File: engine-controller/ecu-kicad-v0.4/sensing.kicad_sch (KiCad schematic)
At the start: 0 parts

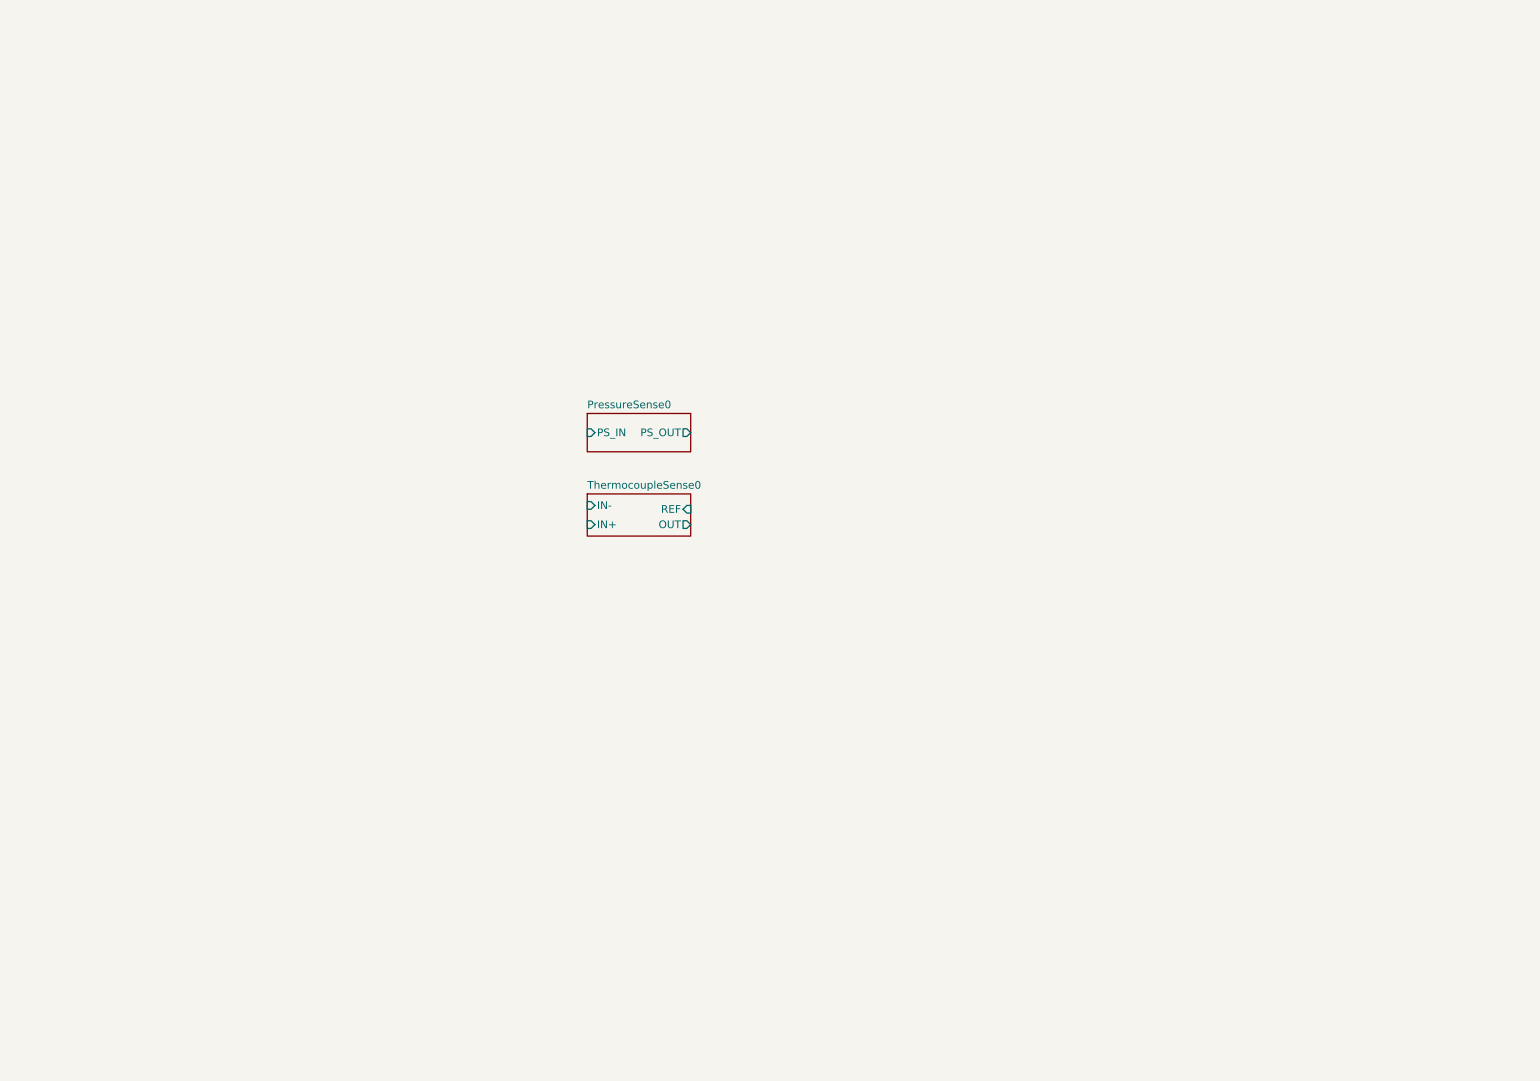
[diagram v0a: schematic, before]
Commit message: Progress on ECU v0.4
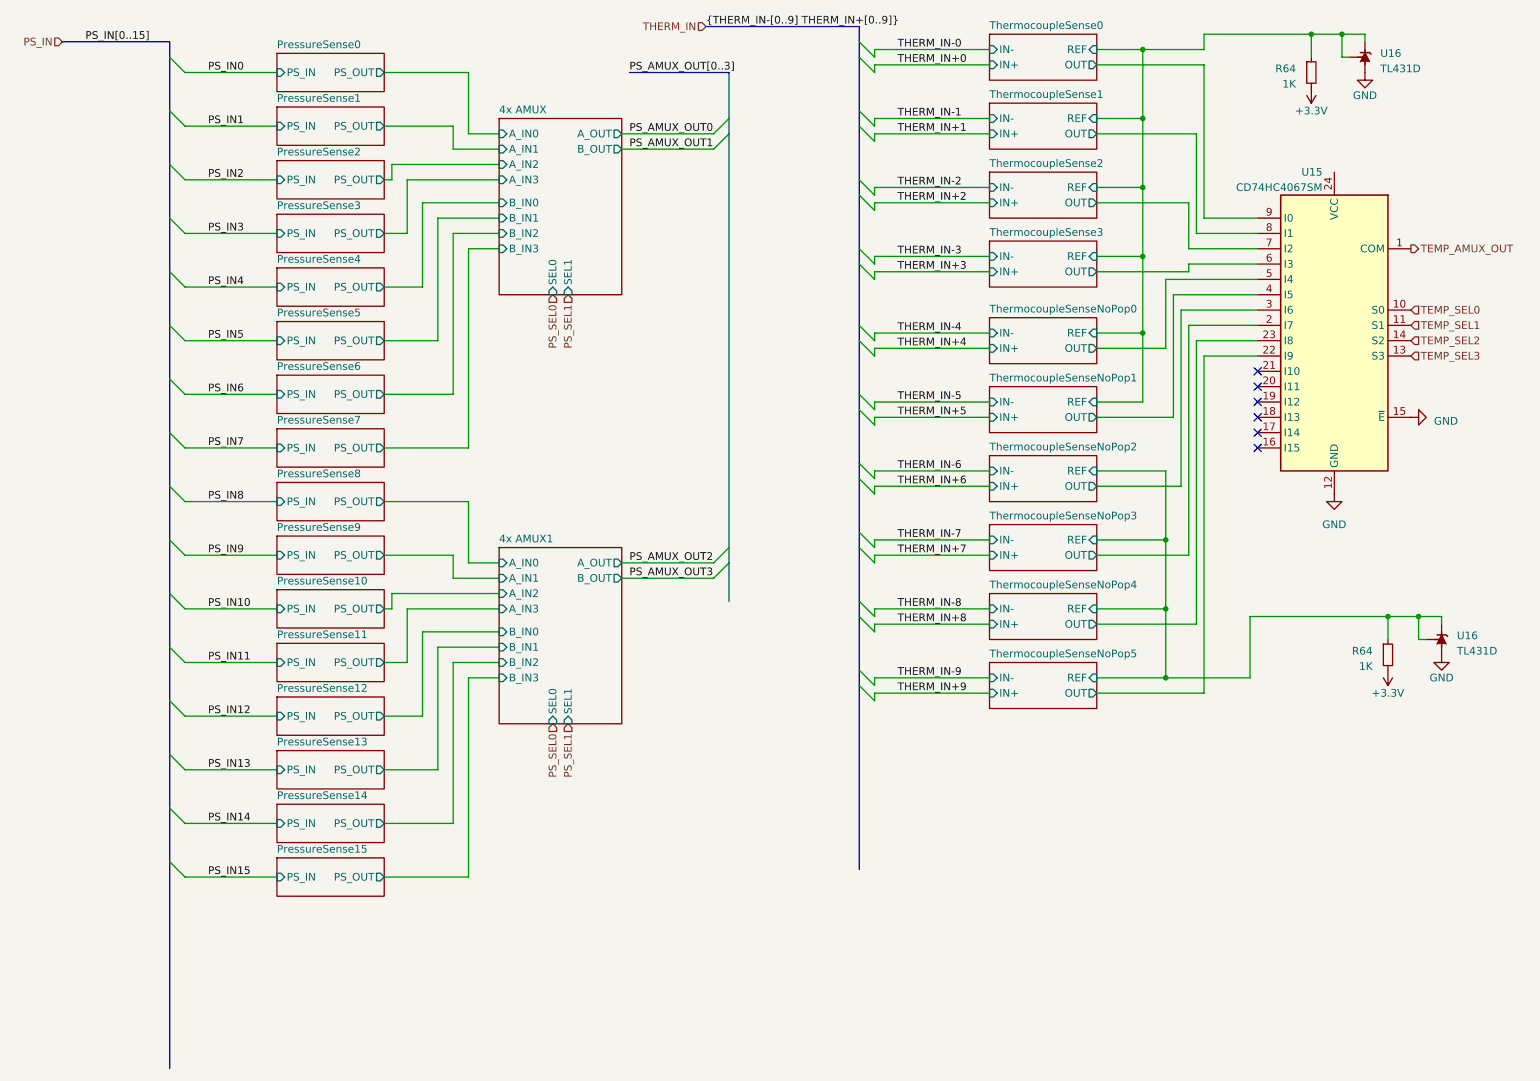
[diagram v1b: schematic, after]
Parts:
- added R64 (x2): 1K, symbol Device:R_Small
- added U15: CD74HC4067SM, Package_SO:SSOP-24_5.3x8.2mm_P0.65mm, symbol 74xx:CD74HC4067SM
- added U16 (x2): TL431D, Package_SO:SOIC-8_3.9x4.9mm_P1.27mm, symbol Reference_Voltage:TL431D
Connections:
- net ThermocoupleSense0/OUT: now also U15.9 (I0)
- net ThermocoupleSense0/REF: now also R64.1, U16.1 (K), U16.8 (REF)
- new net +3.3V: R64.2, R64.2
- new net GND: U15.12 (GND), U15.15 (~{E}), U16.2 (A), U16.2 (A), U16.3 (A), U16.3 (A), U16.6 (A), U16.6 (A), U16.7 (A), U16.7 (A)
- new net TEMP_AMUX_OUT: U15.1 (COM)
- new net TEMP_SEL0: U15.10 (S0)
- new net TEMP_SEL1: U15.11 (S1)
- new net TEMP_SEL2: U15.14 (S2)
- new net TEMP_SEL3: U15.13 (S3)
- new net ThermocoupleSense1/OUT: U15.8 (I1)
- new net ThermocoupleSense2/OUT: U15.7 (I2)
- new net ThermocoupleSense3/OUT: U15.6 (I3)
- new net ThermocoupleSenseNoPop0/OUT: U15.5 (I4)
- new net ThermocoupleSenseNoPop1/OUT: U15.4 (I5)
- new net ThermocoupleSenseNoPop2/OUT: U15.3 (I6)
- new net ThermocoupleSenseNoPop2/REF: R64.1, U16.1 (K), U16.8 (REF)
- new net ThermocoupleSenseNoPop3/OUT: U15.2 (I7)
- new net ThermocoupleSenseNoPop4/OUT: U15.23 (I8)
- new net ThermocoupleSenseNoPop5/OUT: U15.22 (I9)
- no-connect marks 0 -> 6
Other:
- added sheet 4x AMUX (4x_amux.kicad_sch)
- added sheet 4x AMUX1 (4x_amux.kicad_sch)
- added sheet PressureSense1 (pressure_sense.kicad_sch)
- added sheet PressureSense10 (pressure_sense.kicad_sch)
- added sheet PressureSense11 (pressure_sense.kicad_sch)
- added sheet PressureSense12 (pressure_sense.kicad_sch)
- added sheet PressureSense13 (pressure_sense.kicad_sch)
- added sheet PressureSense14 (pressure_sense.kicad_sch)
- added sheet PressureSense15 (pressure_sense.kicad_sch)
- added sheet PressureSense2 (pressure_sense.kicad_sch)
- added sheet PressureSense3 (pressure_sense.kicad_sch)
- added sheet PressureSense4 (pressure_sense.kicad_sch)
- added sheet PressureSense5 (pressure_sense.kicad_sch)
- added sheet PressureSense6 (pressure_sense.kicad_sch)
- added sheet PressureSense7 (pressure_sense.kicad_sch)
- added sheet PressureSense8 (pressure_sense.kicad_sch)
- added sheet PressureSense9 (pressure_sense.kicad_sch)
- added sheet ThermocoupleSense1 (thermocouple_sense.kicad_sch)
- added sheet ThermocoupleSense2 (thermocouple_sense.kicad_sch)
- added sheet ThermocoupleSense3 (thermocouple_sense.kicad_sch)
- added sheet ThermocoupleSenseNoPop0 (thermocouple_sense_no_pop.kicad_sch)
- added sheet ThermocoupleSenseNoPop1 (thermocouple_sense_no_pop.kicad_sch)
- added sheet ThermocoupleSenseNoPop2 (thermocouple_sense_no_pop.kicad_sch)
- added sheet ThermocoupleSenseNoPop3 (thermocouple_sense_no_pop.kicad_sch)
- added sheet ThermocoupleSenseNoPop4 (thermocouple_sense_no_pop.kicad_sch)
- added sheet ThermocoupleSenseNoPop5 (thermocouple_sense_no_pop.kicad_sch)
